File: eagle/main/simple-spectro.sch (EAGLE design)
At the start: 51 parts, among them CON1 BAT, CON2 SPI, CON3 SPI, IC1 32U4, IC2 MCP73831T, IC3 MCP1703-33, IC4 DMP1045U or DMG2302, U1 TMP75DGK, X1 8MHz, X2 MINI-USB

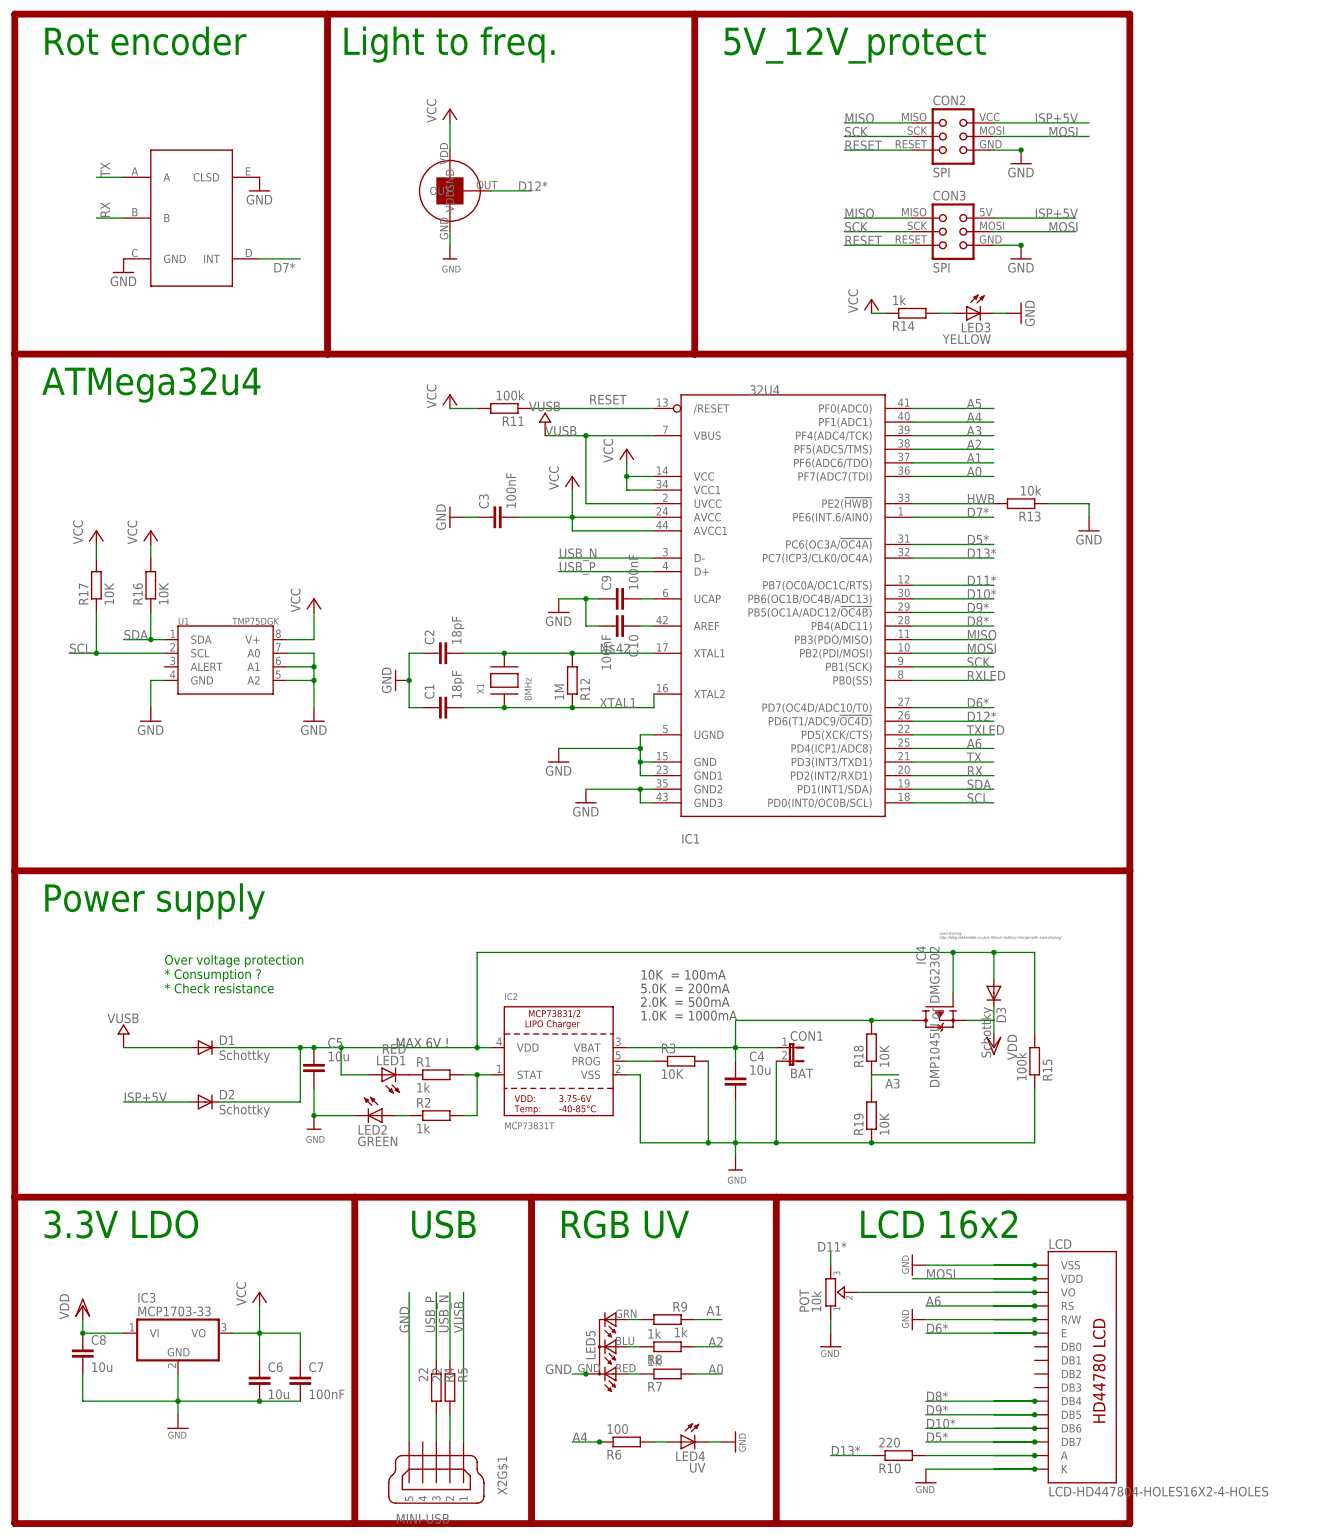
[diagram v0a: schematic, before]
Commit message: working on vibration
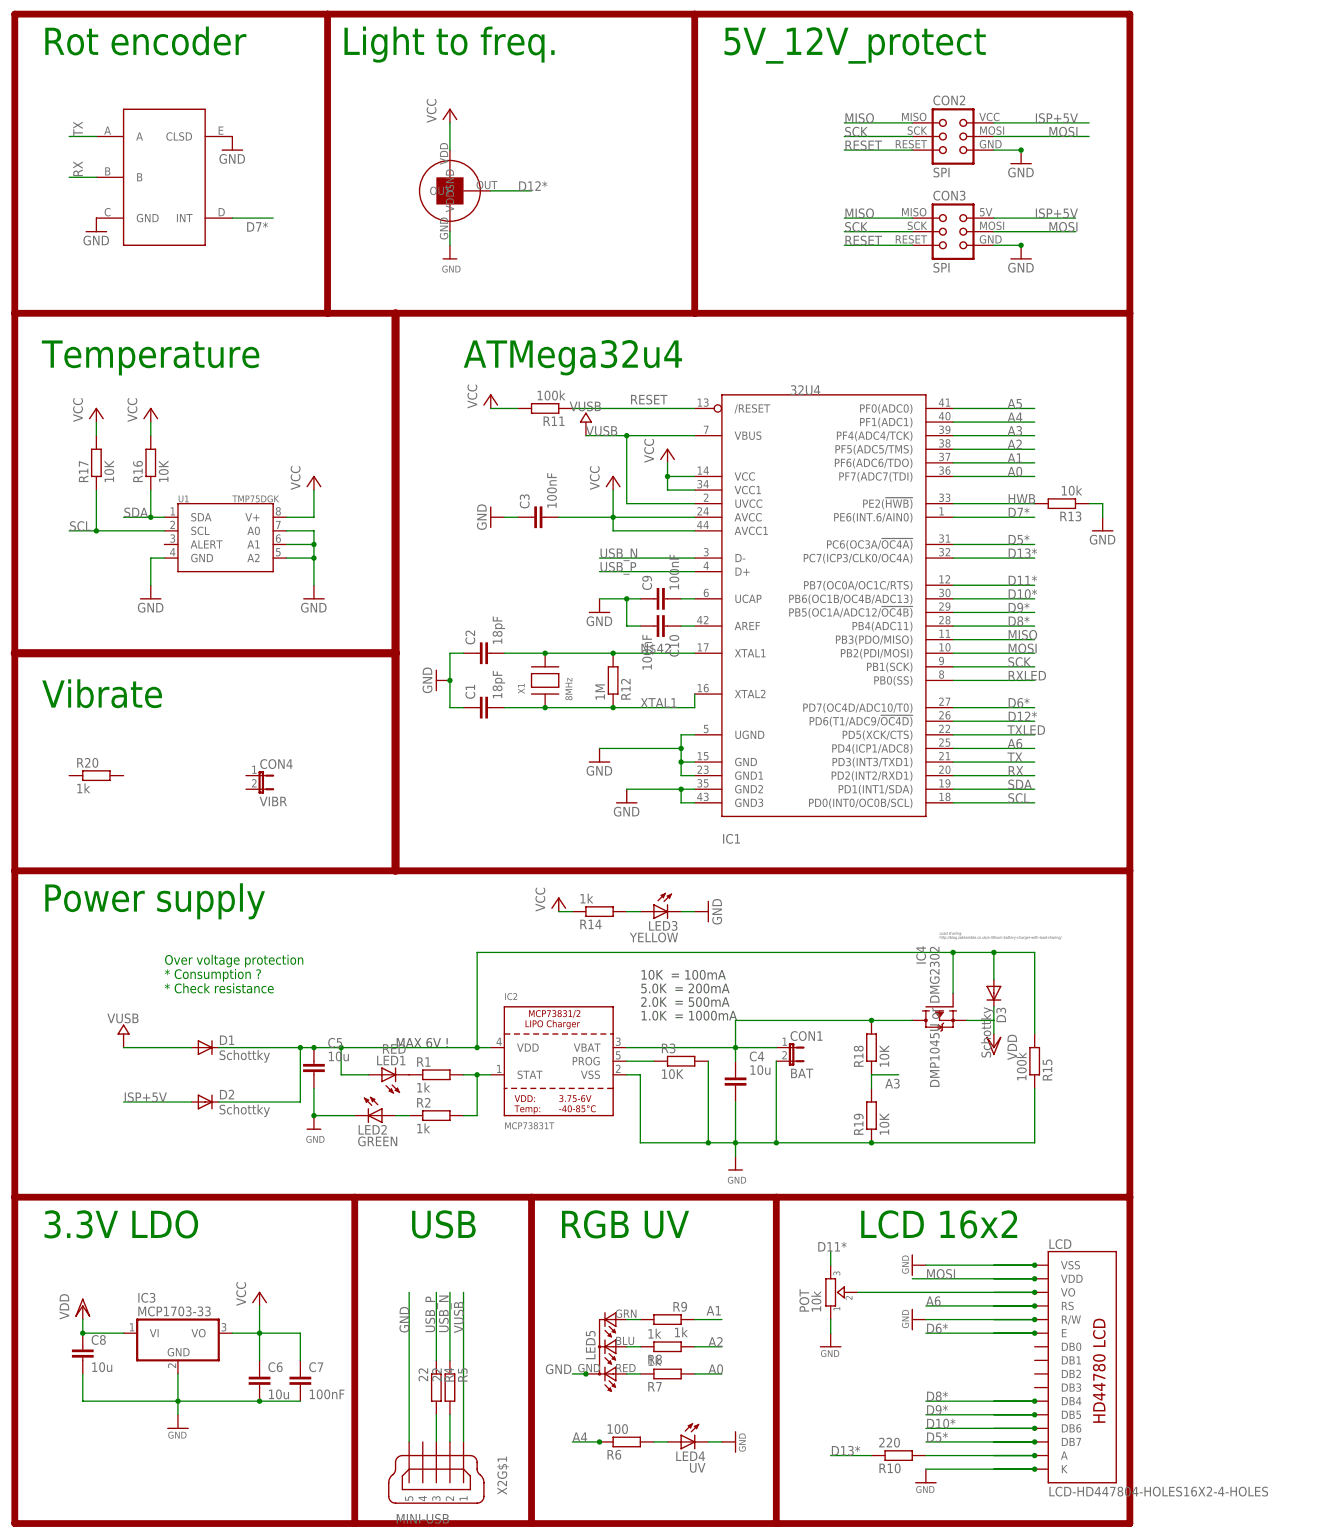
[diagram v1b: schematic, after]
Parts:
- added CON4: VIBR, jumper:JP1E
- added R20: 1k, rcl:R-EU_M1206
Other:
- note added: "Temperature"
- note added: "Vibrate"
- moved on the sheet: C1, C10, C2, C3, C9, IC1, LED3, R11, R12, R13, R14, R16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
